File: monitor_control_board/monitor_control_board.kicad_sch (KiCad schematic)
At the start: 21 parts, among them J2 Conn_01x08_Male, J3 Conn_01x08_Male, J5 Conn_01x05_Male, J6 Conn_01x05_Male, SW1 SW_Push, SW2 SW_Push, SW3 SW_Push, SW4 SW_Push, SW5 SW_Push, SW6 SW_Push, U1 TSSP58038

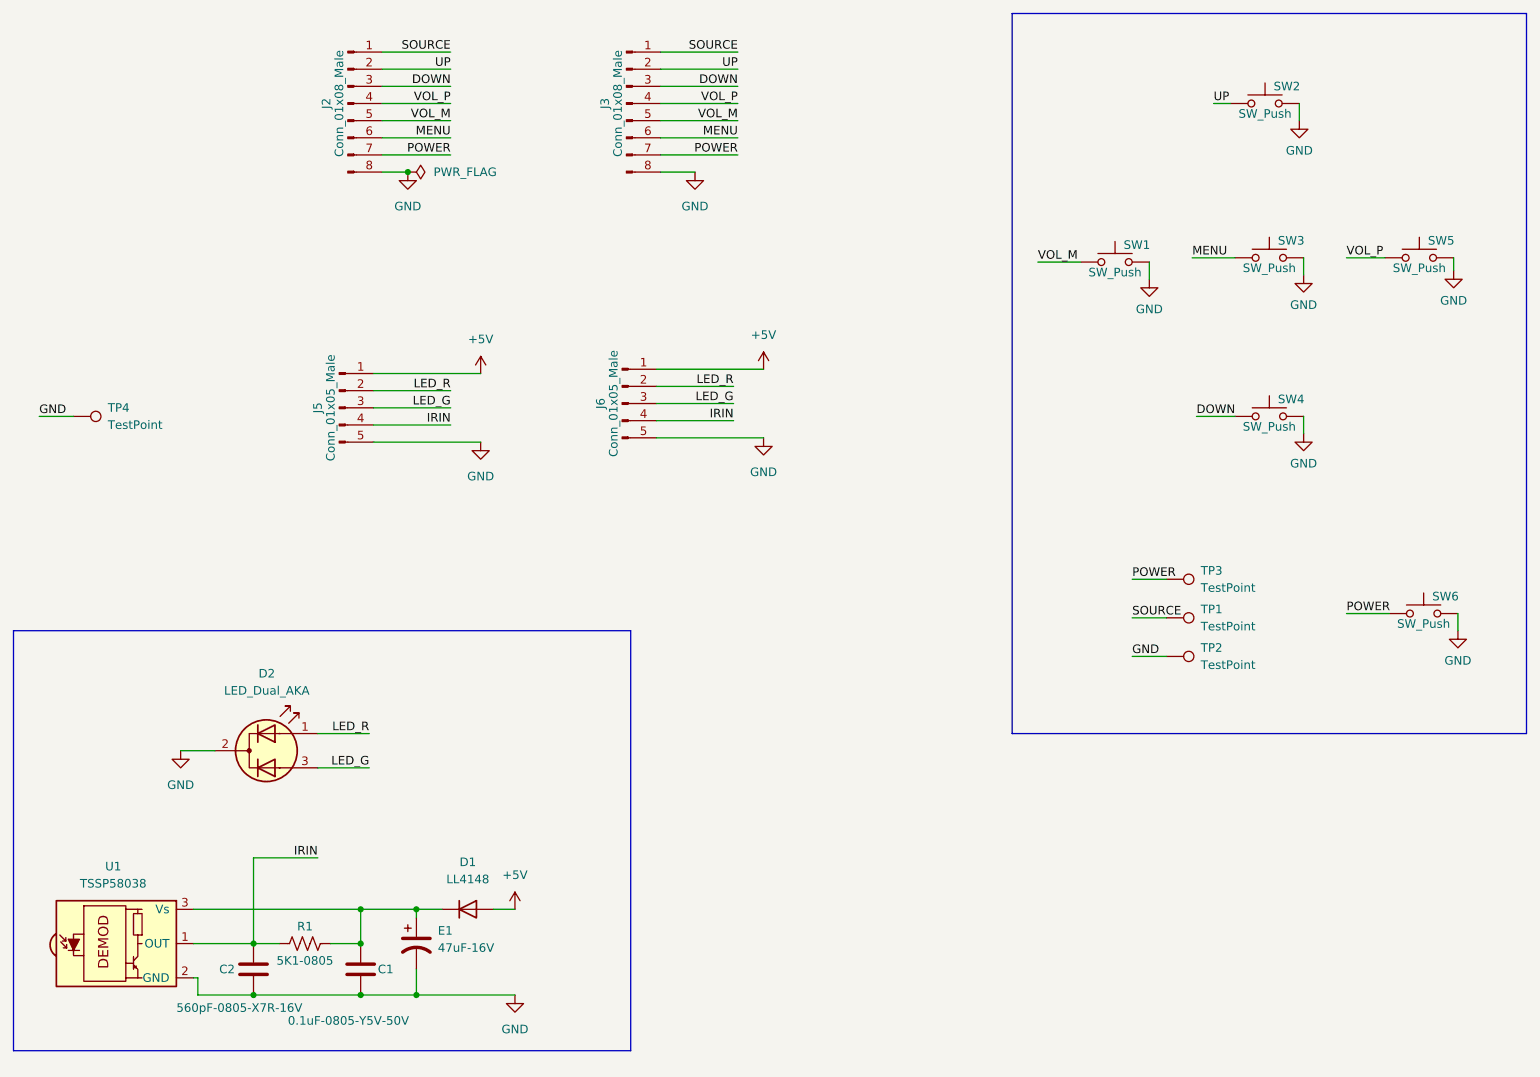
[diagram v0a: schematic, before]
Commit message: PCB 배선 최적화
Signed-off-by: Ju, Gyeong-min <jcmh74@gmail.com>
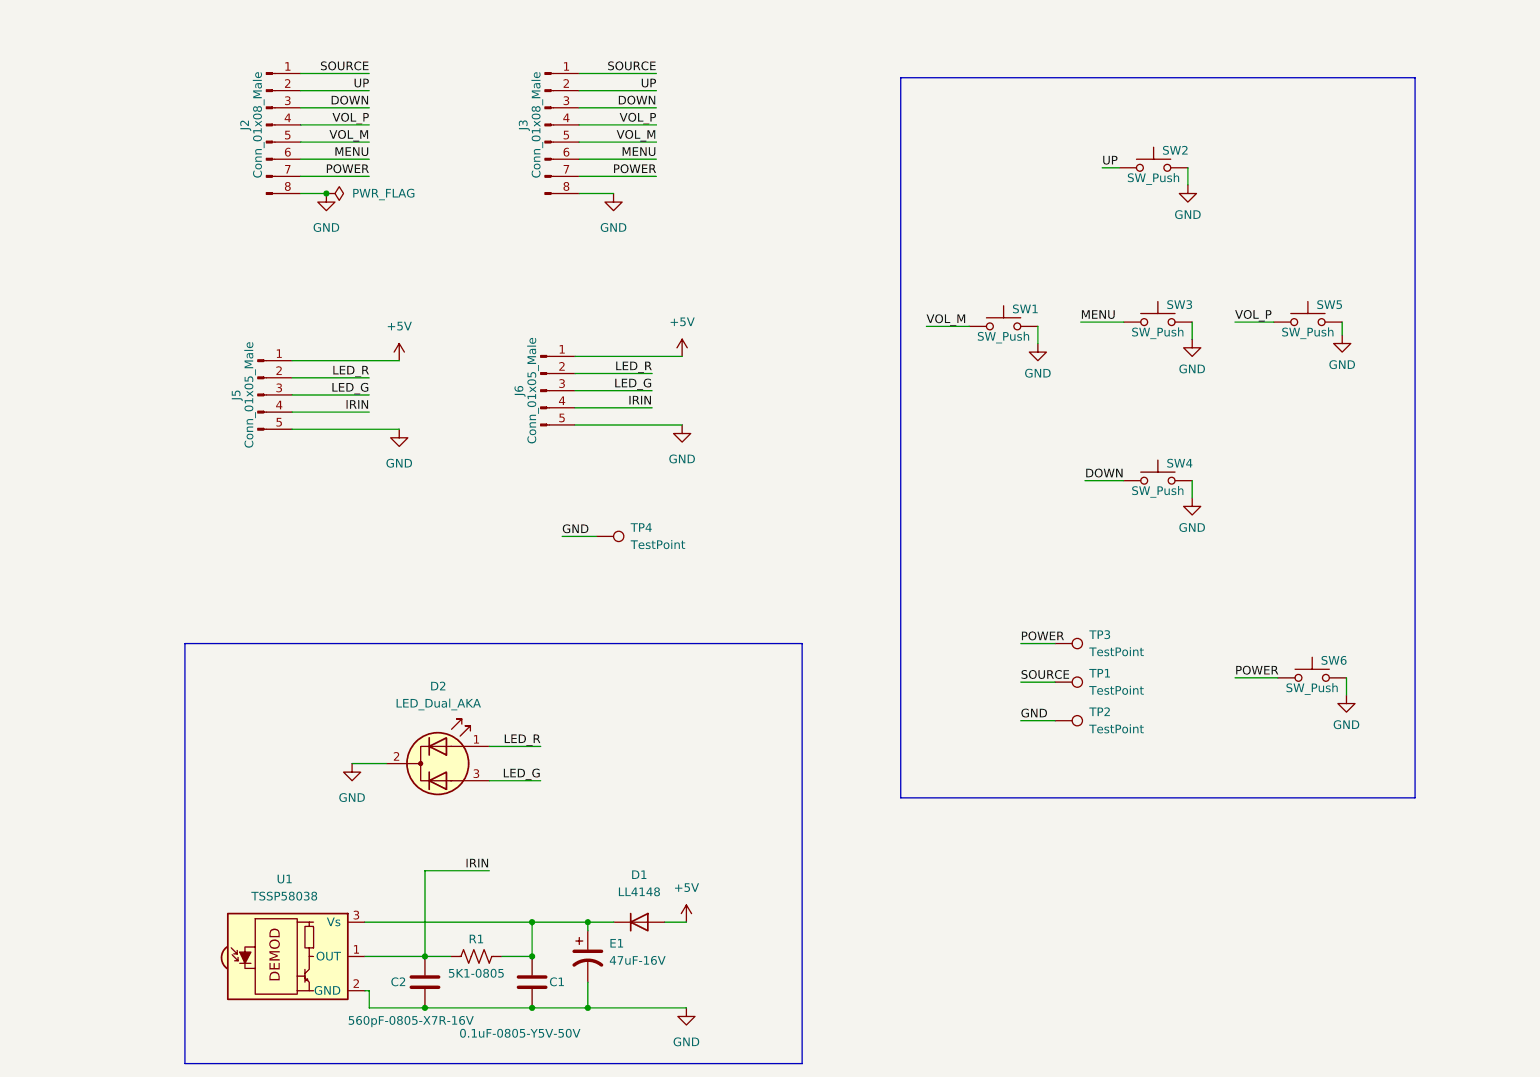
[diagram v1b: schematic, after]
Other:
- moved on the sheet: C1, C2, D1, D2, E1, J2, J3, J5, J6, R1, SW1, SW2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
